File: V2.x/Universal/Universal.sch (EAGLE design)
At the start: 34 parts, among them IC1 Atmega 328-P, IC2 MCP2515, IC3 LM340MP-05, Q1 8MHz, Q2 16MHz

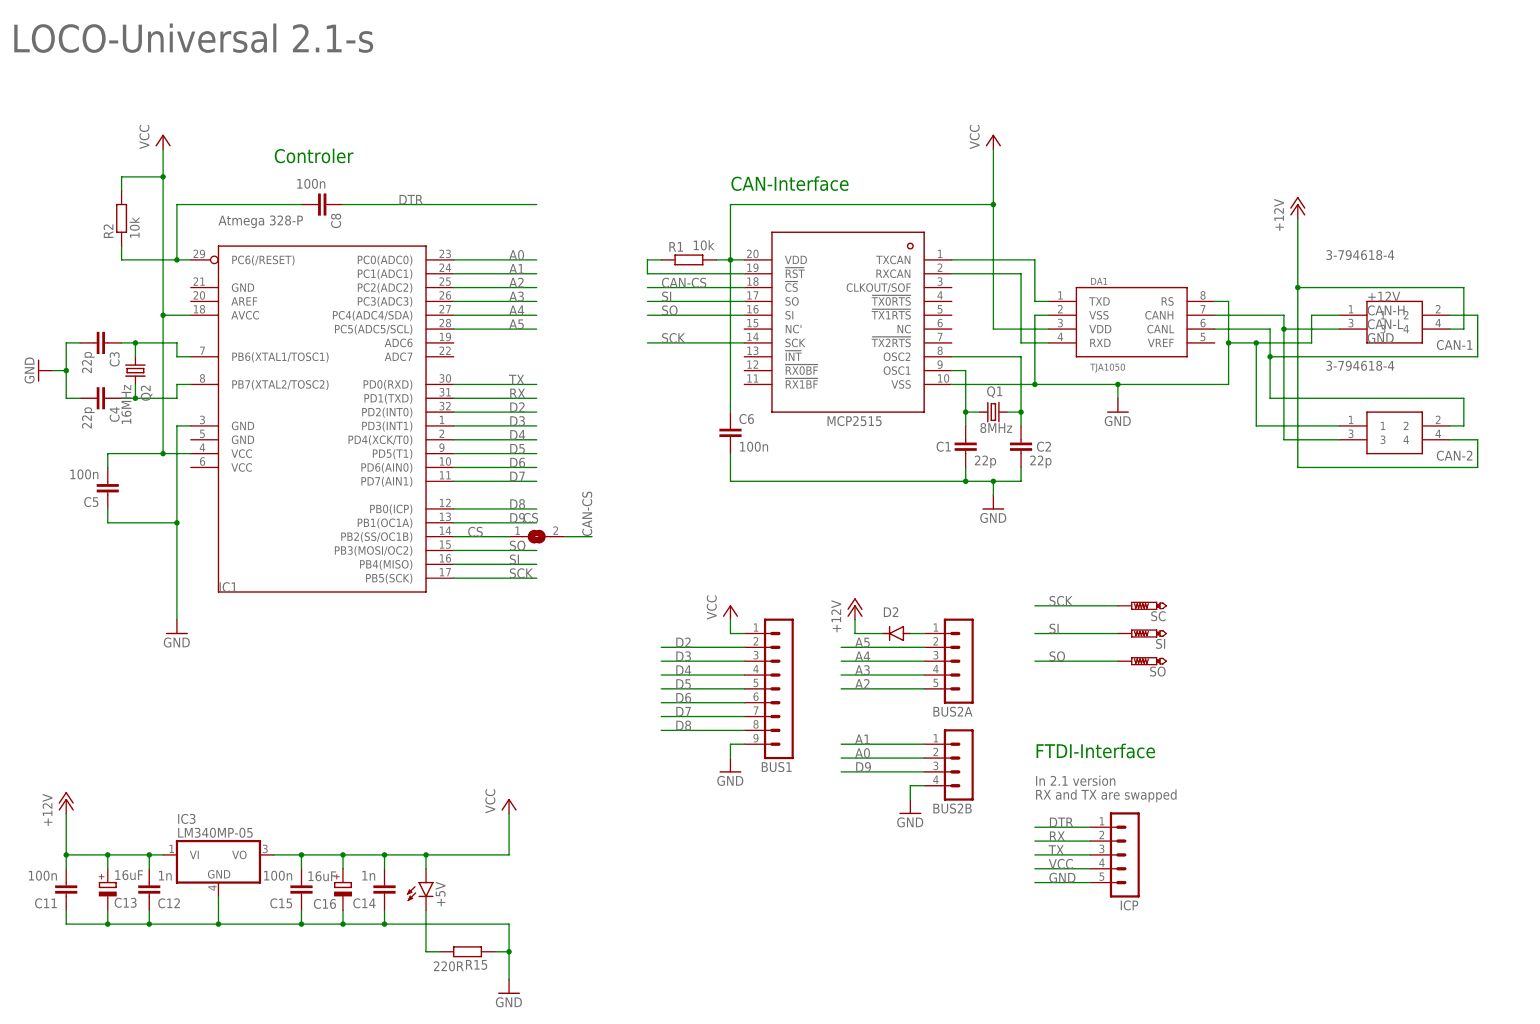
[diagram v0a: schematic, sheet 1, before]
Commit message: initial
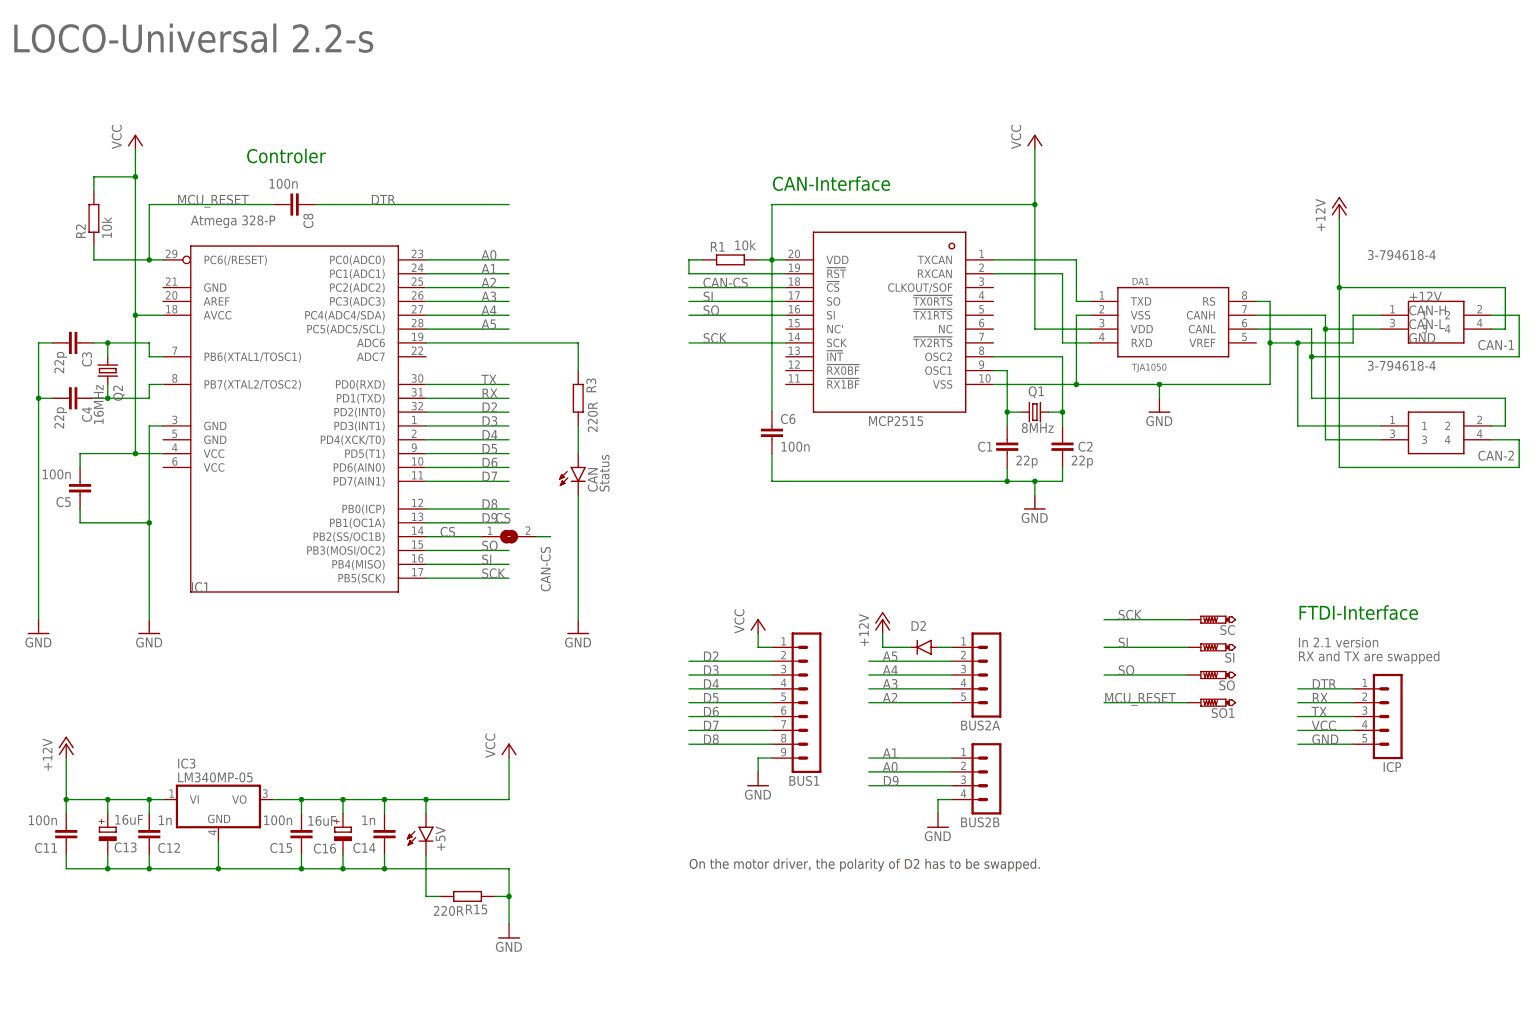
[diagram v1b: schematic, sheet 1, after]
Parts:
- added CAN: Status, led:LEDSML0603
- added R3: 220R, rcl:R-EU_MELF0102W
- added SO1: PTR1B1,27, testpad:PTR1B1,27
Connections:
- removed net N$15: C8.2, IC1.PC6(/RESET), R2.1
- new net MCU_RESET: C8.2, IC1.PC6(/RESET), R2.1, SO1.TP
- new net N$1: IC1.ADC6, R3.1
- new net N$3: CAN.A, R3.2
- net GND: now also CAN.C
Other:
- note added: "LOCO-Universal 2.2-s"
- note added: "On the motor driver, the polarity of D2 has to be swapped."
- note removed: "LOCO-Universal 2.1-s"
- moved on the sheet: +5V, BUS1, BUS2A, BUS2B, C1, C11, C12, C13, C14, C15, C16, C2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
